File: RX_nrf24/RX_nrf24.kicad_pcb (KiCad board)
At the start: 2 copper layers, 58.5 x 30 mm, 46 parts, among them J1 USB_B_Micro, J2 Conn_01x03_Male, J3 Conn_Coaxial, J4 Conn_01x10_Male, J5 Conn_01x04_Female, J6 Conn_01x06_Male, J7 Conn_01x10_Male, J8 Conn_01x10_Male, SW1 SW_Push, U1 USBLC6-2SC6, U2 MCP1700-3302E_SOT23, U3 STM32F103C8Tx, U5 nRF24L01P, Y1 Crystal_GND24, Y2 Crystal_GND24

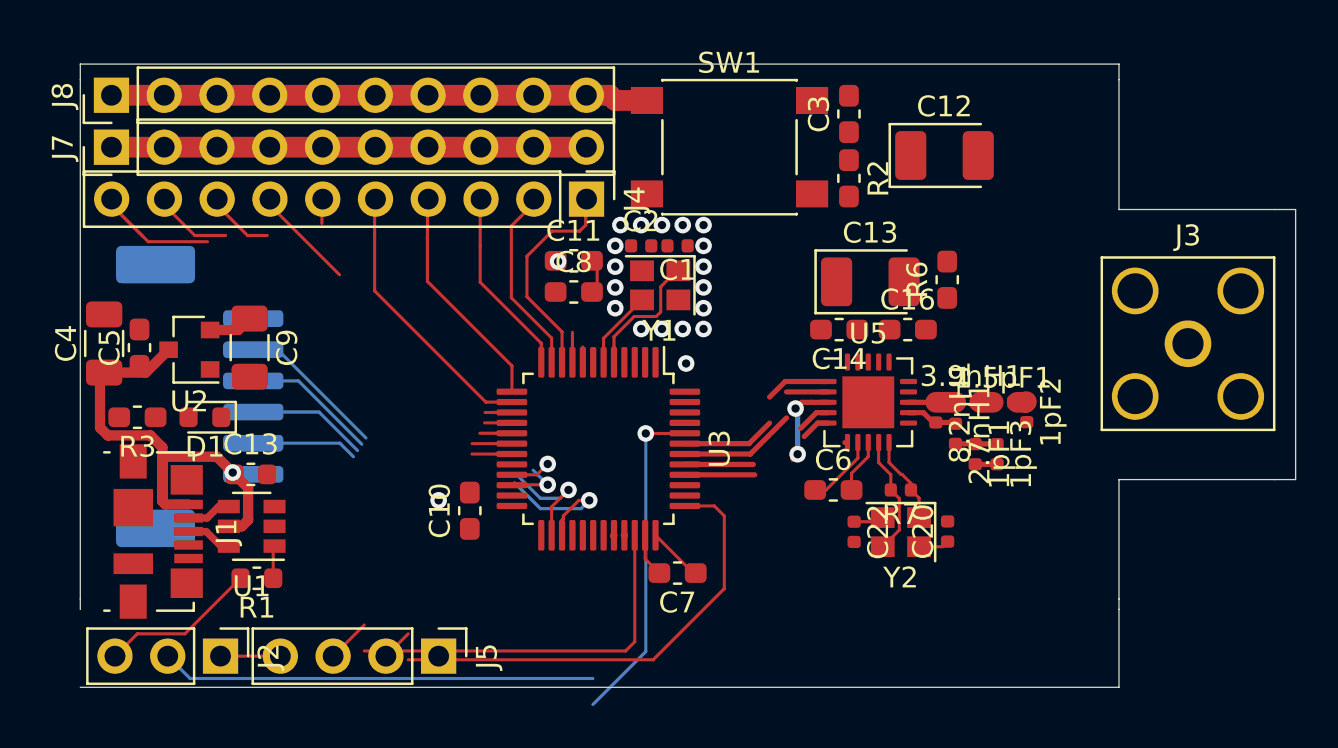
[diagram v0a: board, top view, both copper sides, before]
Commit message: add alot
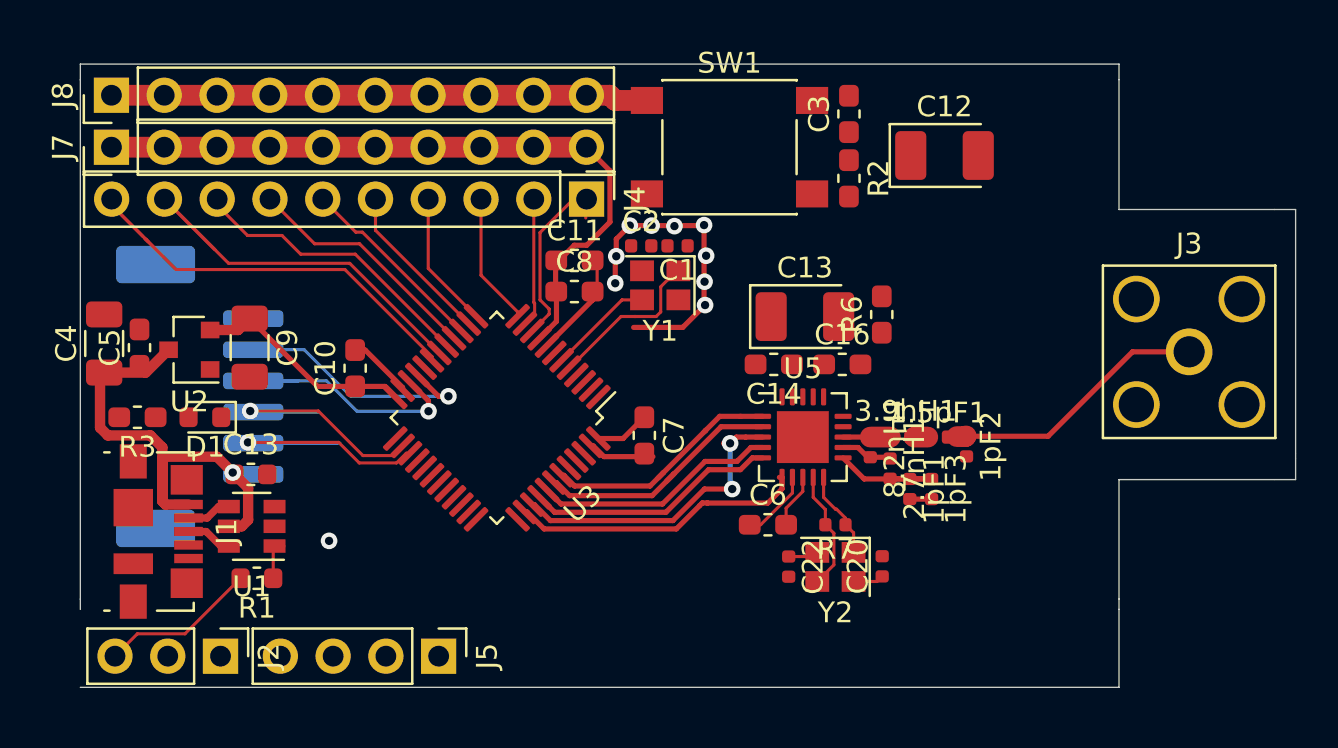
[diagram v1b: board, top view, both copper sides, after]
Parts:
- moved C10 8.81 mm to (163.2, 101.1)
- moved C7 6.82 mm to (177.2, 104.4), turned to 270 degrees
- moved U3 5.11 mm to (170.1, 103.5), turned to 225 degrees
- moved 1.5pF1 3.57 mm to (191.3, 104.5)
- moved 1pF1 3.57 mm to (189.9, 107.0)
- moved 1pF3 3.57 mm to (191.0, 107.0)
- moved 2.7nH1 3.57 mm to (189.0, 106.0)
- moved 3.9nH1 3.57 mm to (189.5, 104.5)
- moved 8.2nH1 3.57 mm to (188.0, 104.9)
- moved C13 3.57 mm to (184.9, 98.7)
- moved C14 3.57 mm to (183.4, 101.0)
- moved C16 3.57 mm to (186.7, 101.0)
- moved C20 3.57 mm to (188.6, 110.7)
- moved C22 3.57 mm to (184.1, 110.7)
- moved C6 3.57 mm to (183.1, 108.7)
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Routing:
- net BOOT0: track 36.9 -> 0.00 mm, vias 1 -> 0
- net SWCLK: track 23.8 -> 0.00 mm
- net SWDIO: track 20.5 -> 0.00 mm
- net GND: track 36.8 -> 55.3 mm, vias 7 -> 10
- net +3V3: track 40.2 -> 58.7 mm, vias 1 -> 0
- net IRQ: track 0.13 -> 14.2 mm
- net P9: track 6.27 -> 19.7 mm
- net RF_out: track 0.46 -> 12.9 mm
- net P10: track 10.3 -> 22.2 mm
- net SCK: track 4.87 -> 15.1 mm
- net P8: track 5.36 -> 13.9 mm
- net MISO: track 4.78 -> 12.1 mm
- net MOSI: track 4.92 -> 11.8 mm
- net P6: track 3.11 -> 9.30 mm
- net P7: track 6.12 -> 11.6 mm
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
